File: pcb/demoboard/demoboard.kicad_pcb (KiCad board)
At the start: 2 copper layers, 68.6 x 48.3 mm, 34 parts, among them J1 BTN, J10 Conn_01x15, J11 Servo2, J12 TEMP, J13 MOT_A, J14 MOT_B, J15 CAP_T, J16 ANALOG, J17 7SEG1, J18 7SEG2, J19 STEPPER1, J2 BAT, J20 STEPPER2, J21 BITS, J22 OLED, J23 Servo3, J24 LIGHT, J3 Conn_01x15, J4 Conn_01x04, J5 Conn_01x15, J6 WSLED, J8 Conn_01x15, J9 Servo1, U2 L293D, U3 PCF8574, U4 ULN2803A

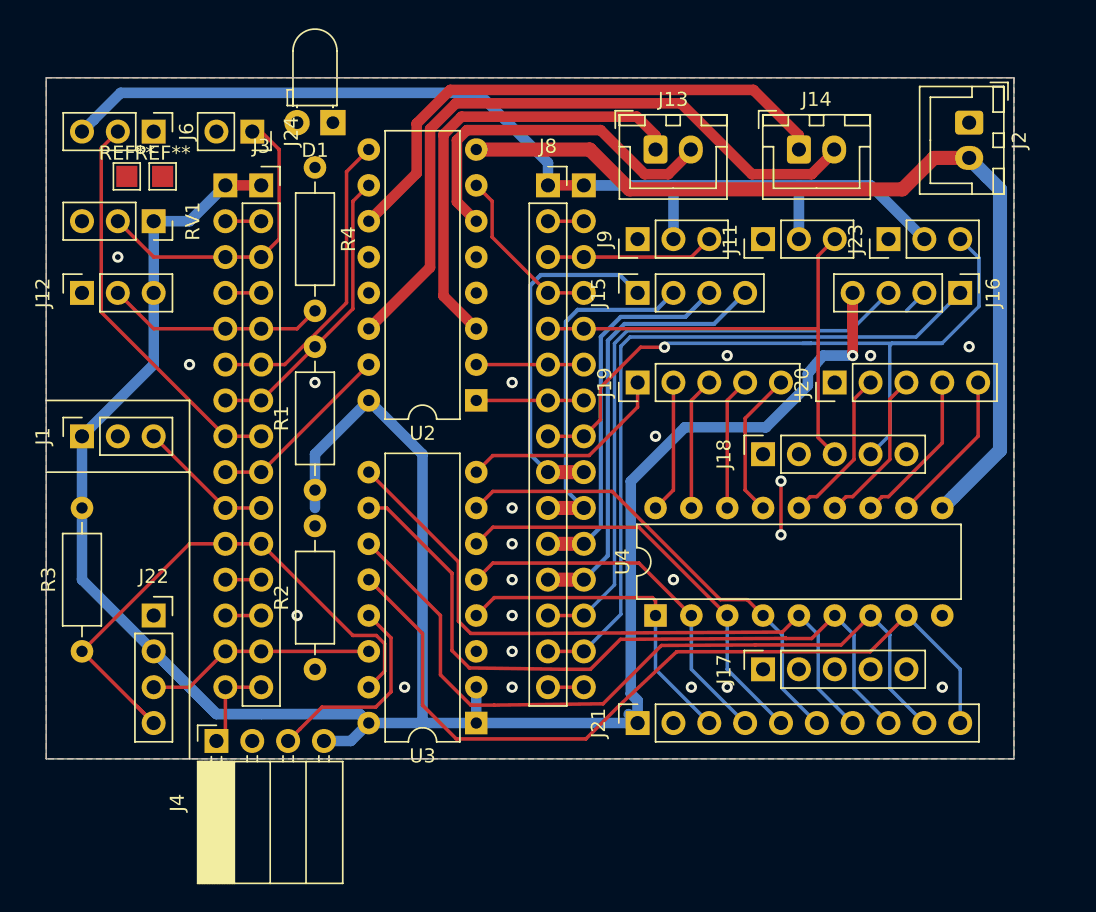
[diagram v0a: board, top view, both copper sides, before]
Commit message: PCB 0.1
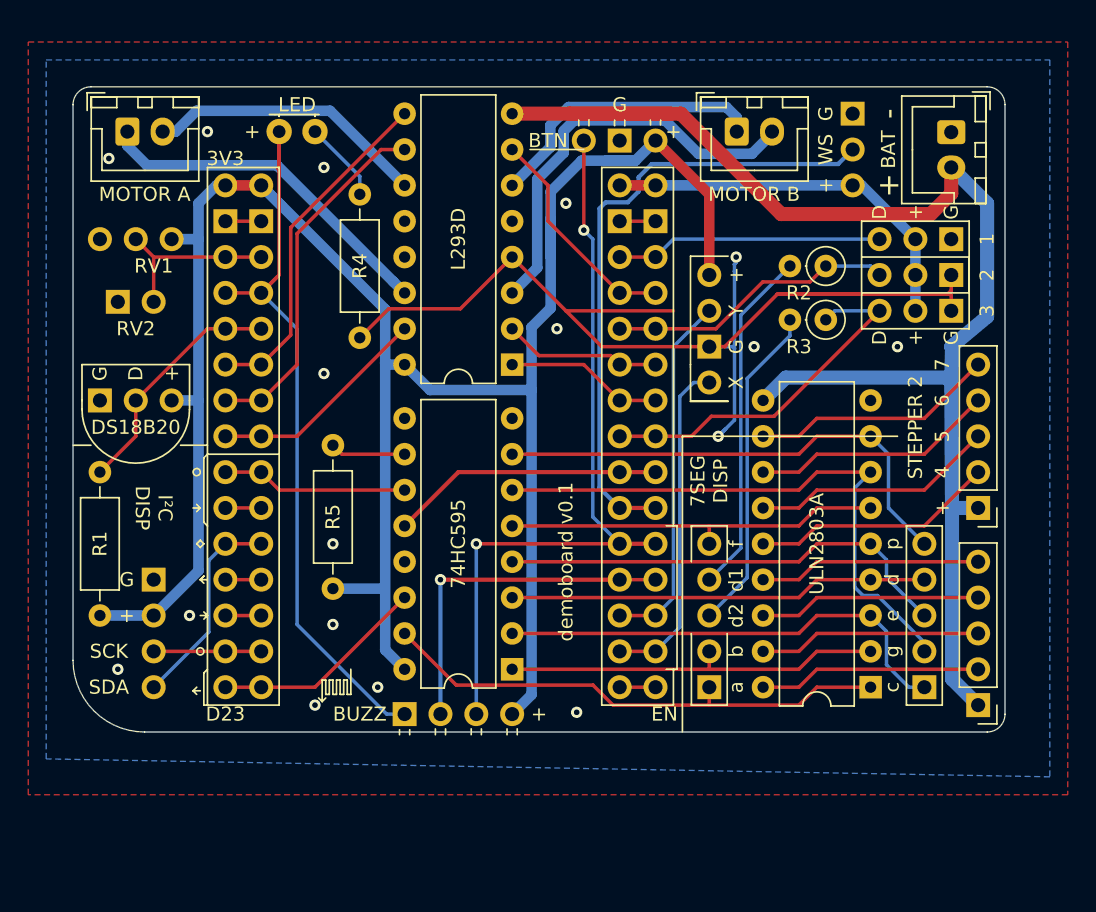
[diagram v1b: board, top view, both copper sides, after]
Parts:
- removed J15: CAP_T, Connector_PinSocket_2.54mm:PinSocket_1x04_P2.54mm_Vertical
- removed J21: BITS, Connector_PinSocket_2.54mm:PinSocket_1x10_P2.54mm_Vertical
- removed REF** (x2): TestPoint_Pad_1.5x1.5mm, TestPoint:TestPoint_Pad_1.5x1.5mm
- removed U3: PCF8574, Package_DIP:DIP-16_W7.62mm
- added R5: 4K7, Resistor_THT:R_Axial_DIN0207_L6.3mm_D2.5mm_P10.16mm_Horizontal, F.Cu at (83.8, 99.7)
- added U1: 74HC595, Package_DIP:DIP-16_W7.62mm, F.Cu at (96.5, 115.6)
- J1: footprint Connector_PinSocket_2.54mm:PinSocket_1x03_P2.54mm_Vertical -> Connector_PinSocket_2.54mm:PinSocket_1x03_P2.54mm_Horizontal
- J10, J3, J5, J8: footprint Connector_PinSocket_2.54mm:PinSocket_1x15_P2.54mm_Vertical -> plain:PlainPinSocket_1x15_P2.54mm_Vertical
- J11, J23, J6, J9: footprint Connector_PinHeader_2.54mm:PinHeader_1x03_P2.54mm_Vertical -> plain:PlainPinHeader_1x03_P2.54mm_Vertical
- J12, RV1: footprint Connector_PinSocket_2.54mm:PinSocket_1x03_P2.54mm_Vertical -> plain:PlainPinSocket_1x03_P2.54mm_Vertical
- J17, J18: footprint Connector_PinSocket_2.54mm:PinSocket_1x05_P2.54mm_Vertical -> plain:PlainPinSocket_1x05_P2.54mm_Vertical
- J22: footprint Connector_PinSocket_2.54mm:PinSocket_1x04_P2.54mm_Vertical -> plain:PlainPinSocket_1x04_P2.54mm_Vertical
- J24: value LIGHT -> RV2; footprint Connector_PinSocket_2.54mm:PinSocket_1x02_P2.54mm_Vertical -> plain:PlainPinSocket_1x02_P2.54mm_Vertical
- R2, R3: value 4K7 -> 220R; footprint Resistor_THT:R_Axial_DIN0207_L6.3mm_D2.5mm_P10.16mm_Horizontal -> Resistor_THT:R_Axial_DIN0207_L6.3mm_D2.5mm_P2.54mm_Vertical
- moved R3 57.7 mm to (118.7, 90.8), turned to 180 degrees
- moved J6 49.5 mm to (120.7, 76.2), turned to 0 degrees
- moved J14 47.6 mm to (69.3, 77.5)
- moved R2 46.1 mm to (118.7, 87.0), turned to 180 degrees
- moved J1 45.7 mm to (106.7, 78.1), turned to 270 degrees
- moved J19 33.2 mm to (129.5, 118.1), turned to 180 degrees
- moved J9 22.2 mm to (127.6, 85.1), turned to 270 degrees
- moved J16 18.9 mm to (110.5, 95.2), turned to 180 degrees
- moved R1 17.6 mm to (67.3, 111.8)
- moved J18 16.9 mm to (110.5, 116.8), turned to 180 degrees
- moved U4 16.1 mm to (121.9, 116.8), turned to 180 degrees
- moved J24 13.9 mm to (71.1, 89.5)
- moved J11 13.6 mm to (127.6, 87.6), turned to 270 degrees
- moved J20 13.5 mm to (129.5, 104.1), turned to 180 degrees
- moved J4 13.5 mm to (88.9, 118.7)
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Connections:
- J10 pad 11: /D35 -> /BTN
- J13 pad 1: /MA1Y -> /MA2Y
- J13 pad 2: /MA2Y -> /MA1Y
- J14 pad 1: /MB1Y -> /MB2Y
- J14 pad 2: /MB2Y -> /MB1Y
- J17 pad 1: /B0 -> /B2
- J17 pad 2: /B1 -> /B6
- J17 pad 3: /B2 -> /B4
- J17 pad 5: /B4 -> /B7
- J18 pad 1: /B5 -> /B0
- J18 pad 2: /B6 -> /B1
- J18 pad 3: /D14 -> Net-(J18-Pad3)
- J18 pad 4: /D25 -> Net-(J18-Pad4)
- J18 pad 5: /B7 -> /B5
- J3 pad 10: /BTN -> /D19
- J3 pad 15: /BUZZ -> /D23
- J3 pad 9: /D18 -> /CLK
- J4 pad 1: /BUZZ -> /D2
- J4 pad 2: (no net) -> /D34
- J4 pad 3: /INT -> /BTN
- J5 pad 10: /BTN -> /D19
- J5 pad 15: /BUZZ -> /D23
- J5 pad 9: /D18 -> /CLK
- J6 pad 2: /D5 -> /D32
- J8 pad 11: /D35 -> /BTN
- R2 pad 1: /D22 -> /D14
- R2 pad 2: VCC -> Net-(J18-Pad4)
- R3 pad 1: /D21 -> /D25
- R3 pad 2: VCC -> Net-(J18-Pad3)
- U2 pad 15: /D18 -> /D5
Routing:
- net GND: track 25.8 -> 91.7 mm, vias 22 -> 17
- net /D2: track 2.54 -> 53.6 mm
- net /VIN: track 73.7 -> 27.6 mm
- net /BTN: track 9.72 -> 54.4 mm, vias 0 -> 2
- net VDC: track 64.4 -> 100.9 mm
- net /D25: track 53.8 -> 26.2 mm, vias 1 -> 0
- net /D36: track 50.9 -> 23.8 mm
- net /D35: track 26.7 -> 0.00 mm
- net /D21: track 39.9 -> 14.8 mm
- net Net-(J18-Pad4): track 0.00 -> 24.6 mm
- net /B5: track 51.7 -> 27.2 mm
- net /B7: track 58.5 -> 35.1 mm
- net Net-(J18-Pad3): track 0.00 -> 23.3 mm
- net /MB2Y: track 48.2 -> 25.0 mm
- net /D32: track 24.7 -> 44.6 mm
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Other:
- board size 68.6 x 48.3 mm -> 66 x 45.7 mm
- board text added: "+"
- board text added: "-"
- board text added: "1"
- board text added: "13"
- board text added: "14"
- board text added: "2"
- board text added: "25"
- board text added: "3"
- board text added: "36"
- board text added: "39"
- board text added: "3V"
- board text added: "3V3"
- board text added: "4"
- board text added: "5"
- board text added: "6"
- board text added: "7"
- board text added: "7SEG DISP"
- board text added: "A1Y"
- board text added: "A2Y"
- board text added: "B0"
- board text added: "B1"
- board text added: "B1Y"
- board text added: "B2"
- board text added: "B2Y"
- board text added: "B3"
- board text added: "B4"
- board text added: "B5"
- board text added: "B6"
- board text added: "B7"
- board text added: "BUZZ"
- board text added: "D"
- board text added: "D02"
- board text added: "D1"
- board text added: "D12"
- board text added: "D13"
- board text added: "D14"
- board text added: "D15"
- board text added: "D16"
- board text added: "D17"
- board text added: "D18"
- board text added: "D19"
- board text added: "D2"
- board text added: "D21"
- board text added: "D22"
- board text added: "D23"
- board text added: "D25"
- board text added: "D26"
- board text added: "D27"
- board text added: "D3"
- board text added: "D32"
- board text added: "D33"
- board text added: "D34"
- board text added: "D35"
- board text added: "D36"
- board text added: "D39"
- board text added: "D4"
- board text added: "D5"
- board text added: "DS18B20"
- board text added: "EN"
- board text added: "G"
- board text added: "GND"
- board text added: "I²C DISP"
- board text added: "LED"
- board text added: "MOTOR A"
- board text added: "MOTOR B"
- board text added: "NC"
- board text added: "OE"
- board text added: "P0"
- board text added: "P1"
- board text added: "P2"
- board text added: "P3"
- board text added: "P4"
- board text added: "P5"
- board text added: "P6"
- board text added: "P7"
- board text added: "RCL"
- board text added: "SCK"
- board text added: "SCL"
- board text added: "SDA"
- board text added: "SER"
- board text added: "SRCLR"
- board text added: "STEPPER 2"
- board text added: "VDC"
- board text added: "VIN"
- board text added: "WS"
- board text added: "X"
- board text added: "Y"
- board text added: "a"
- board text added: "b"
- board text added: "c"
- board text added: "d"
- board text added: "d1"
- board text added: "d2"
- board text added: "demoboard v0.1"
- board text added: "e"
- board text added: "f"
- board text added: "g"
- board text added: "hi"
- board text added: "p"
